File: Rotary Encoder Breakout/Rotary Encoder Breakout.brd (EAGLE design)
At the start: 17.8 x 25.4 mm, 2 parts, among them P1 HDR-4, SW1 SWITCH-ALPS_EC12E_SW

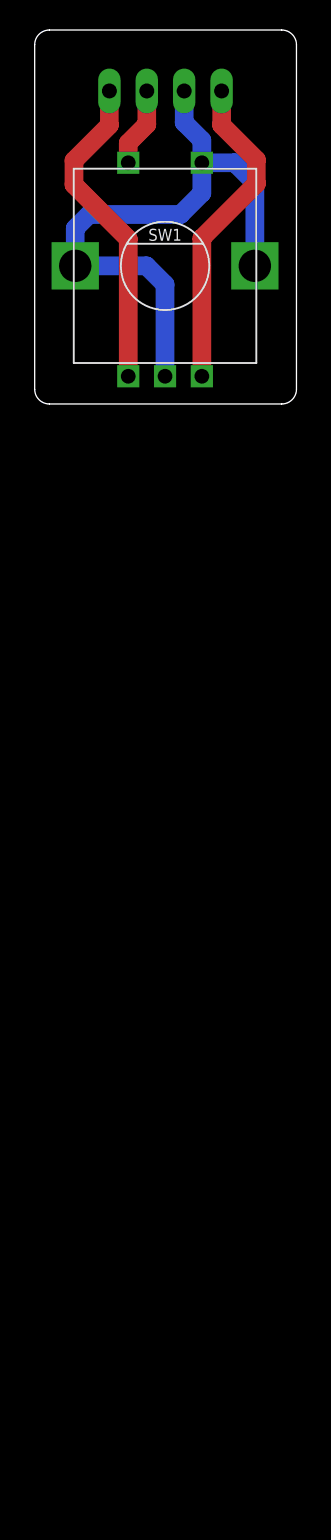
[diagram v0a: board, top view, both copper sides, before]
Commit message: Updated part
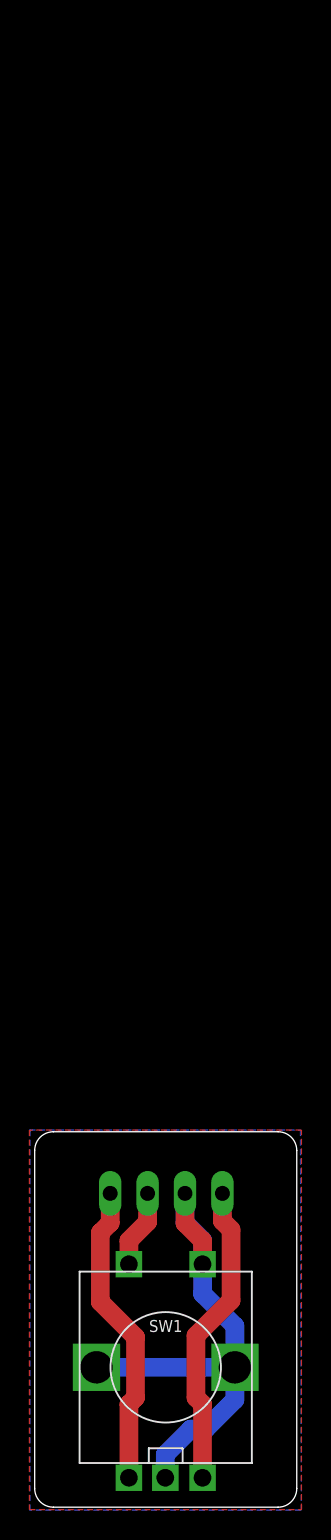
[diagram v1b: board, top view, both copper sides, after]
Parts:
- removed P1: HDR-4, Donnie:HDR-4_VERT
- added H1: HDR-4, Donnie:HDR-4_VERT
- SW1: value SWITCH-ALPS_EC12E_SW -> (none); device Donnie:SWITCH-ALPS_ALPS_EC12E_SW -> LBussy:ACZ11BRXE
- moved SW1 74.8 mm to (8.90, 9.50)
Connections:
- net GND: now also H1.2, SW1.G1, SW1.G2, SW1.S2; no longer P1.2, SW1.1, SW1.2, SW1.E
- net PB: now also H1.3, SW1.S1; no longer P1.3, SW1.D
- net ROTA: now also H1.4; no longer P1.4
- net ROTB: now also H1.1; no longer P1.1
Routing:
- net GND: track 42.2 -> 38.0 mm
- net ROTB: track 21.9 -> 20.7 mm
- net ROTA: track 21.9 -> 20.8 mm
- added copper zone on layer 1, net GND
- added copper zone on layer 16, net GND
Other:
- board size 17.8 x 25.4 mm -> 17.8 x 25.5 mm
